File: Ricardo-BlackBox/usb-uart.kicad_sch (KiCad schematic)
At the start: 9 parts, among them J2 USB_C_Receptacle_USB2.0

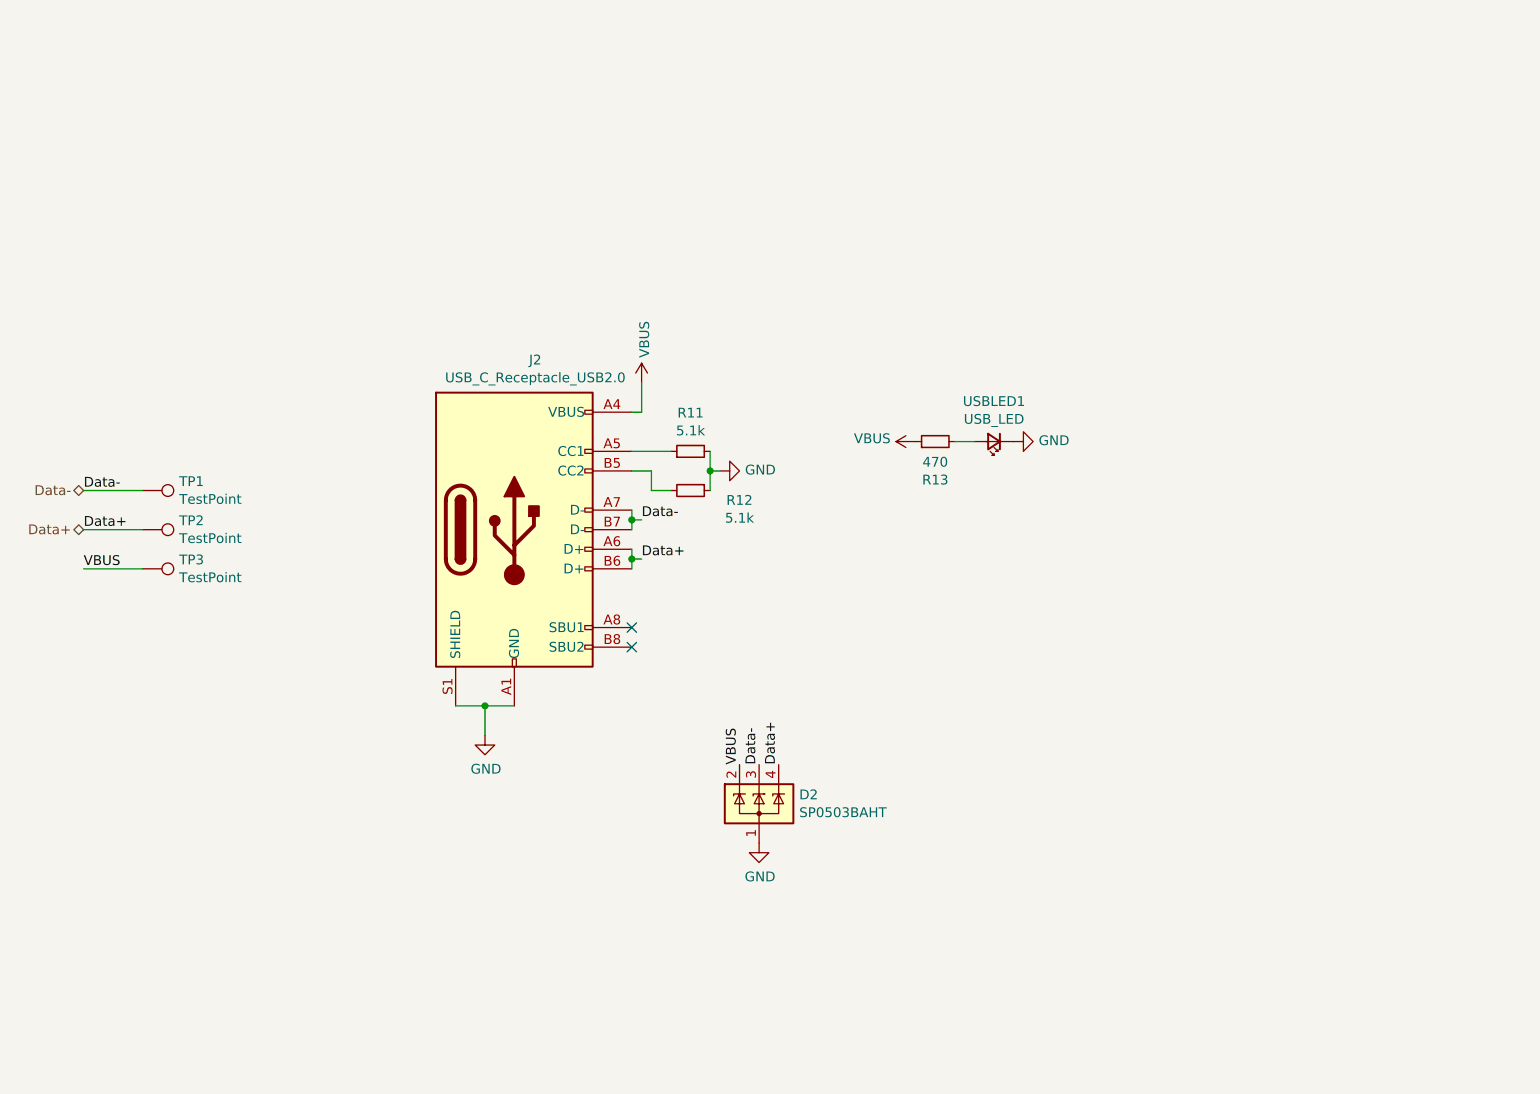
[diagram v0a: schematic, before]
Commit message: AsOf13/12/2022
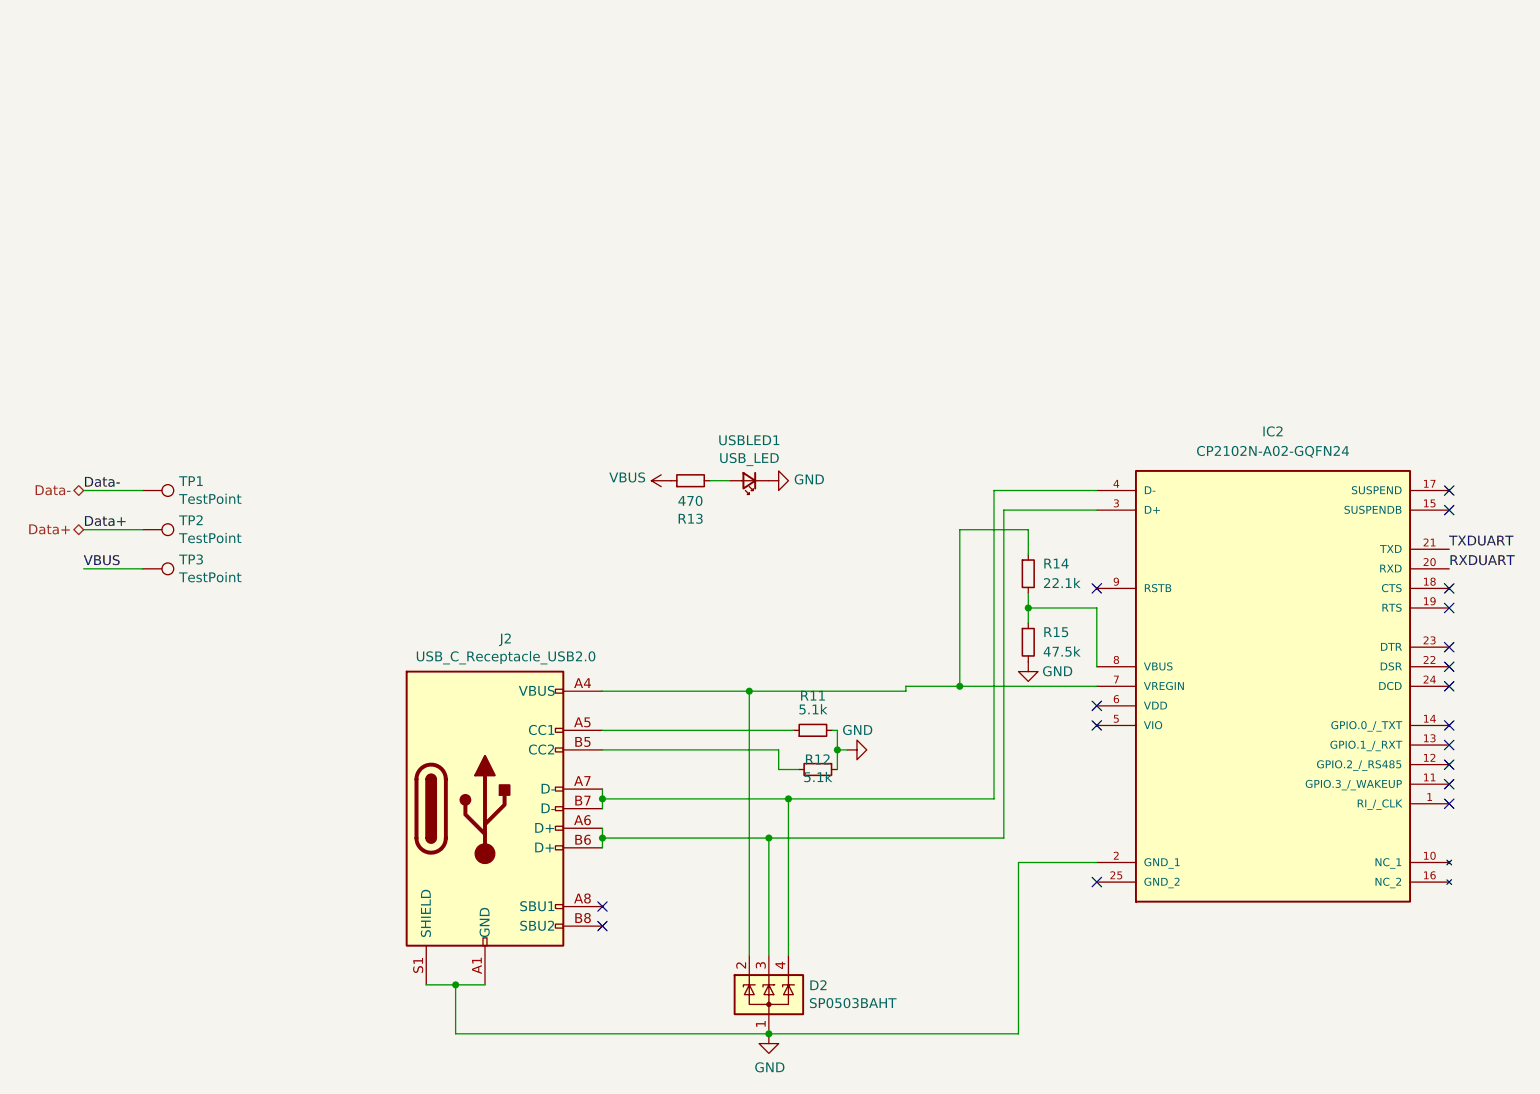
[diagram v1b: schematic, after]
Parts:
- added IC2: CP2102N-A02-GQFN24, symbol iclr:CP2102N-A02-GQFN24
- added R14: 22.1k, Resistor_SMD:R_0402_1005Metric, symbol Device:R_Small
- added R15: 47.5k, Resistor_SMD:R_0402_1005Metric, symbol Device:R_Small
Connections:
- net Data+: no longer D2.4 (K), J2.A6 (D+), J2.B6 (D+)
- net Data-: no longer D2.3 (K), J2.A7 (D-), J2.B7 (D-)
- net GND: now also IC2.2 (GND_1), R15.2
- net VBUS: no longer D2.2 (K), J2.A4 (VBUS), J2.A9 (VBUS), J2.B4 (VBUS), J2.B9 (VBUS)
- new net: D2.2 (K), IC2.7 (VREGIN), J2.A4 (VBUS), J2.A9 (VBUS), J2.B4 (VBUS), J2.B9 (VBUS), R14.1
- new net: D2.3 (K), IC2.3 (D+), J2.A6 (D+), J2.B6 (D+)
- new net: D2.4 (K), IC2.4 (D-), J2.A7 (D-), J2.B7 (D-)
- new net: IC2.8 (VBUS), R14.2, R15.1
- new net RXDUART: IC2.20 (RXD)
- new net TXDUART: IC2.21 (TXD)
- no-connect marks 2 -> 18
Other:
- moved on the sheet: D2, J2, R11, R12, R13, USBLED1

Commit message: AsOf31/01/2023
Schematic should be done, PCB beginning to be done
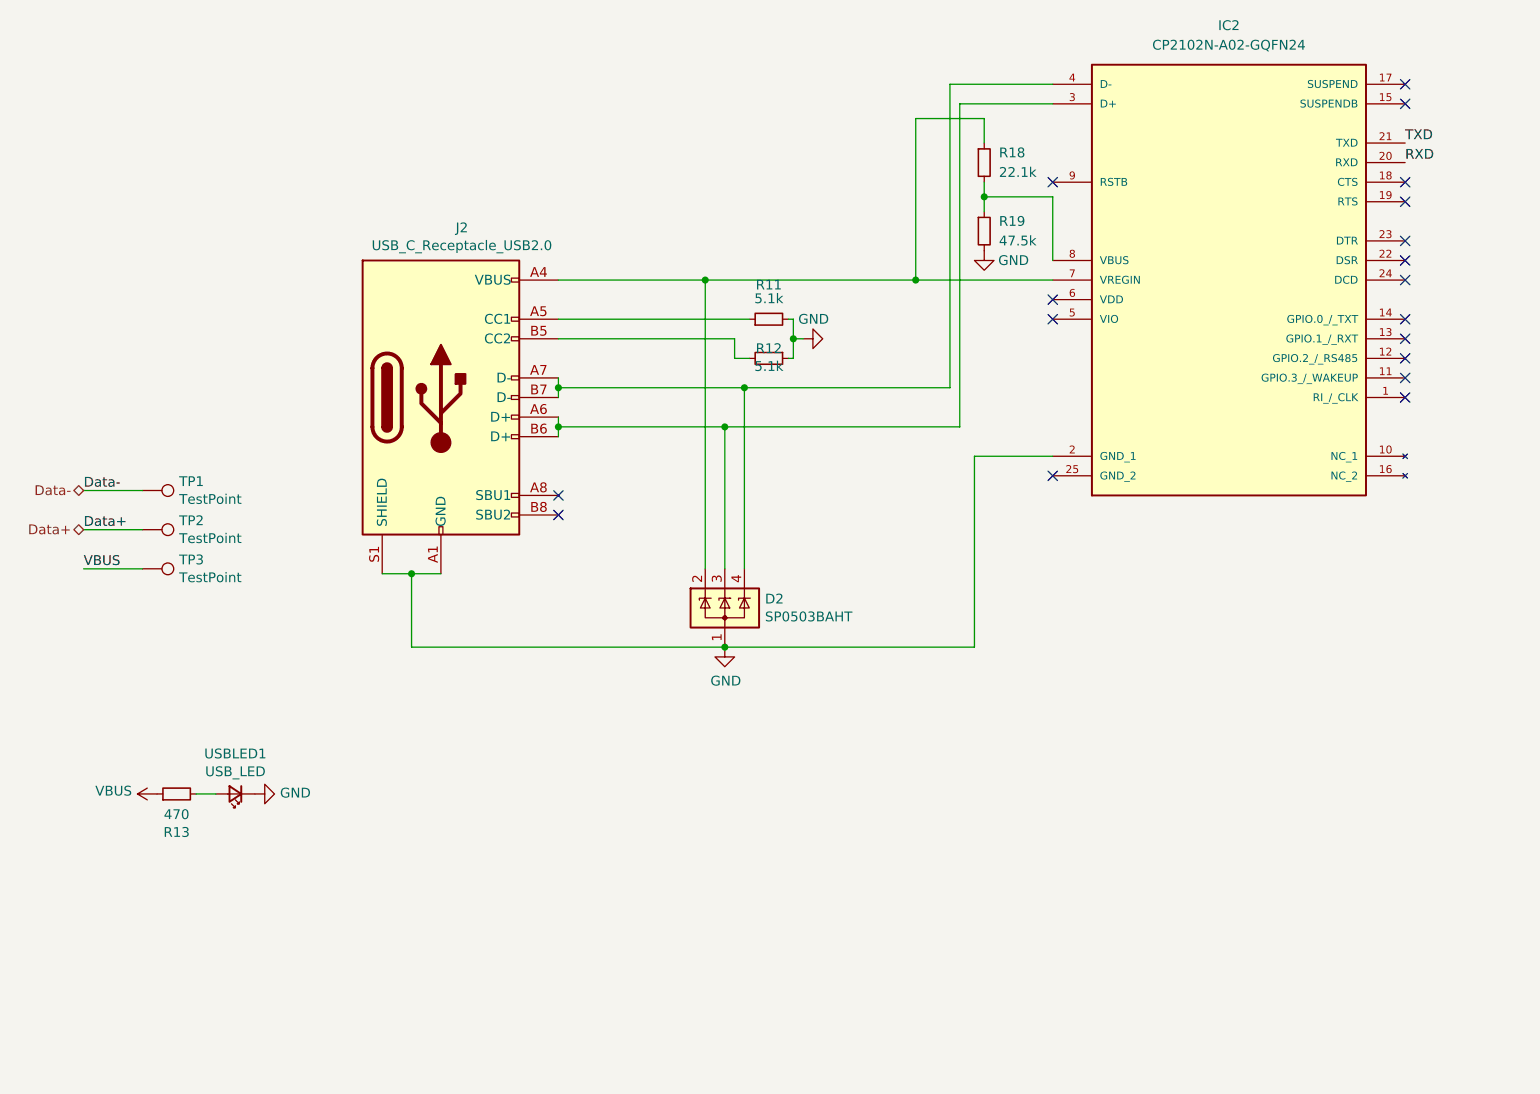
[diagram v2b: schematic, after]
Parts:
- removed R14: 22.1k, Resistor_SMD:R_0402_1005Metric, symbol Device:R_Small
- removed R15: 47.5k, Resistor_SMD:R_0402_1005Metric, symbol Device:R_Small
- added R18: 22.1k, Resistor_SMD:R_0402_1005Metric, symbol Device:R_Small
- added R19: 47.5k, Resistor_SMD:R_0402_1005Metric, symbol Device:R_Small
- IC2: footprint (none) -> iclr:QFN50P400X400X80-25N
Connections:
- net GND: now also R19.2
- net at D2.2 (K), IC2.7 (VREGIN), J2.A4 (VBUS)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: now also R18.1
- net at IC2.8 (VBUS): now also R18.2, R19.1
- net RXDUART renamed RXD
- net TXDUART renamed TXD
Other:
- moved on the sheet: D2, J2, R13, USBLED1
